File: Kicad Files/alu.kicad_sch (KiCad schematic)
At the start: 29 parts, among them U40 SST39SF040, U41 SST39SF040, U42 74LS173, U43 74HC245, U44 74HC245

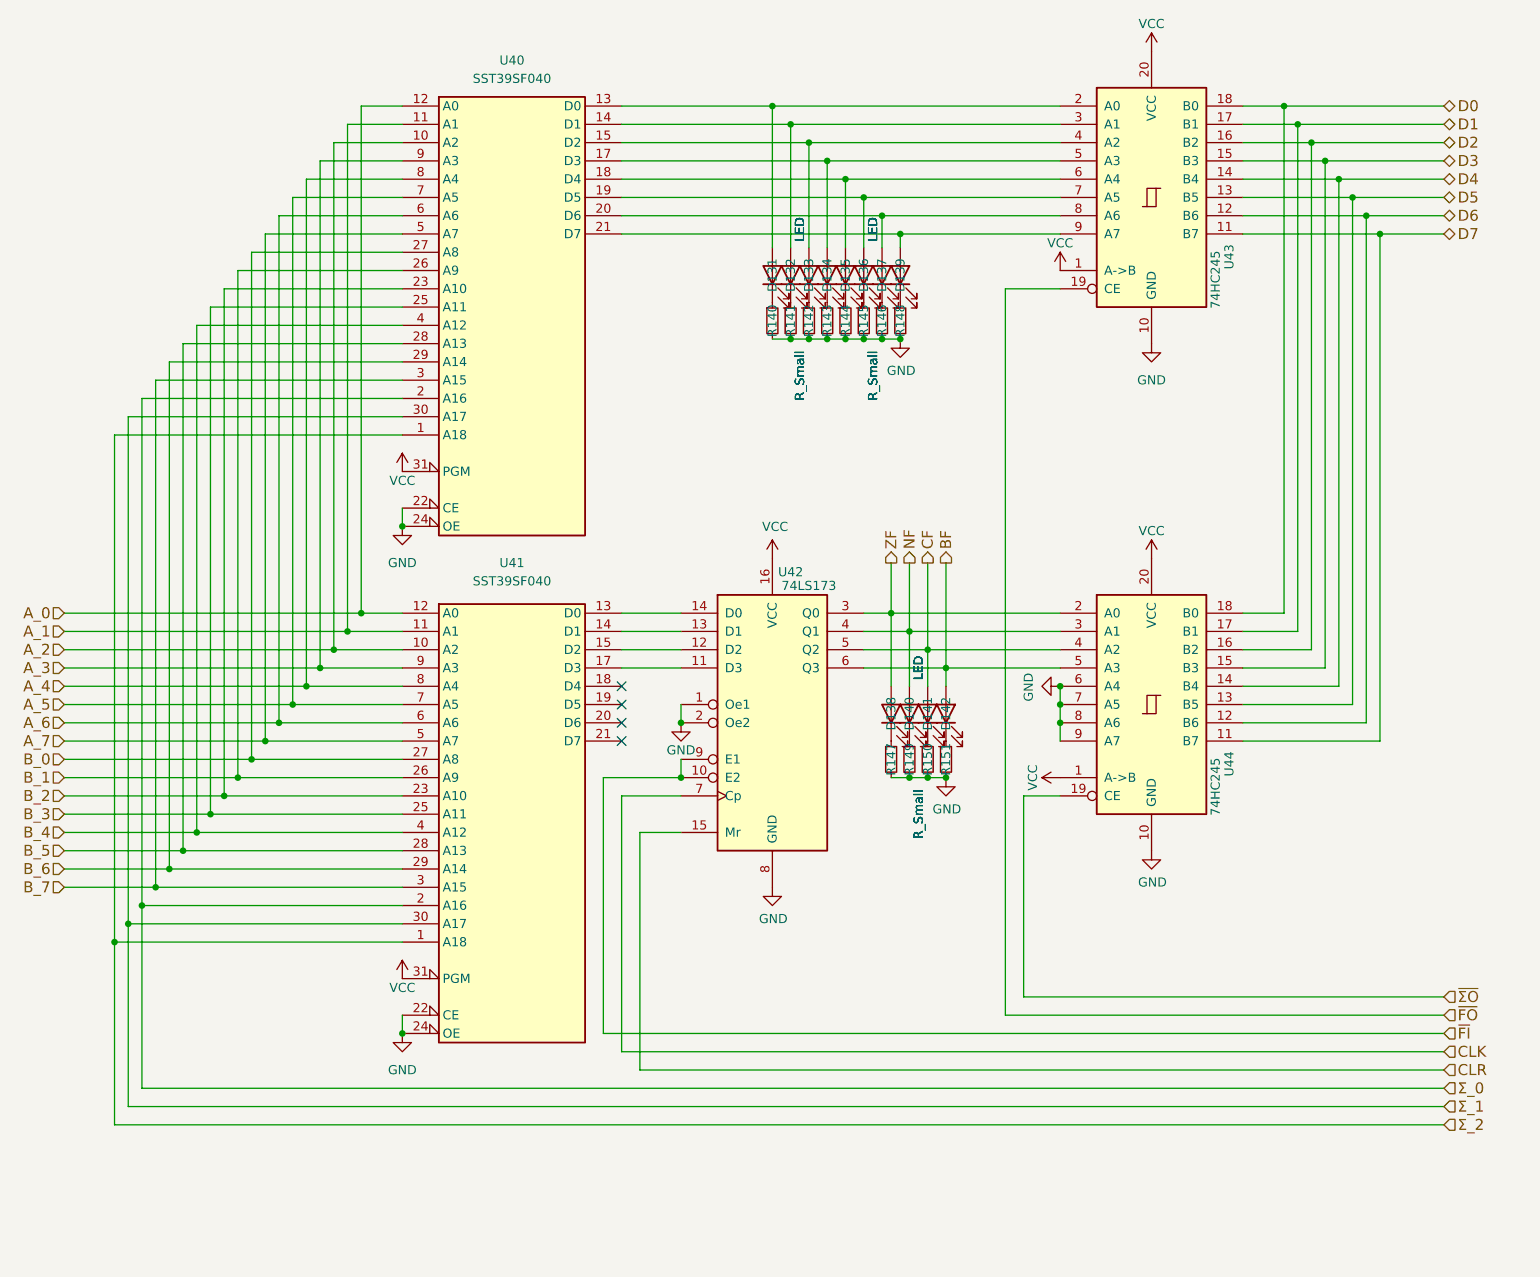
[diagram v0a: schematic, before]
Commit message: update
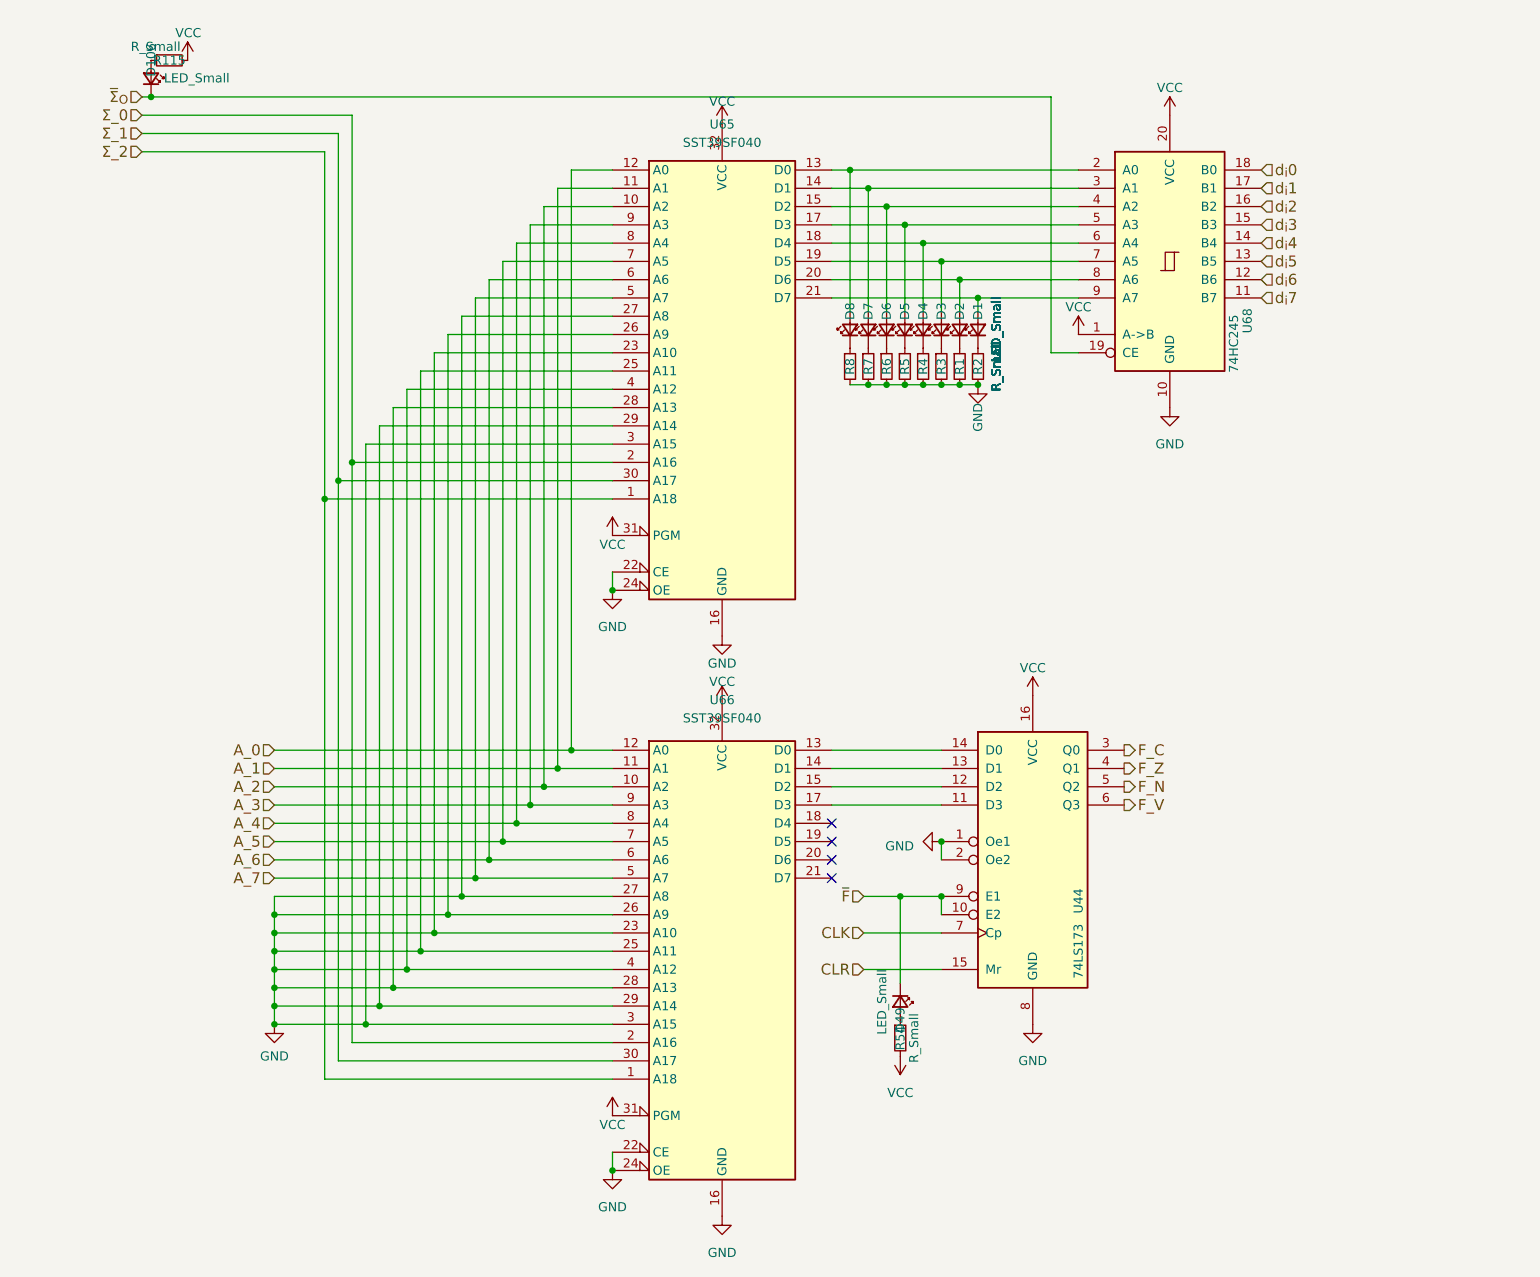
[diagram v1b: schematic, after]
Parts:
- removed D131, D132, D133, D134, D135, D136, D137, D138, D139, D140, D141, D142: LED, symbol Device:LED
- removed R140, R141, R142, R143, R144, R145, R146, R147, R148, R149, R150, R151: R_Small, symbol Device:R_Small
- removed U42: 74LS173, symbol 74xx:74LS173
- removed U44: 74HC245, symbol 74xx:74HC245
- added D1, D106, D2, D3, D4, D49, D5, D6, D7, D8: LED_Small, symbol Device:LED_Small
- added R1, R115, R2, R3, R4, R5, R54, R6, R7, R8: R_Small, symbol Device:R_Small
- added U44: 74LS173, symbol 74xx:74LS173
- renumbered U40 to U65, U41 to U66, U43 to U68
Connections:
- net B_0 is gone; now on net GND: U65.27 (A8), U66.27 (A8)
- net B_1 is gone; now on net GND: U65.26 (A9), U66.26 (A9)
- net B_2 is gone; now on net GND: U65.23 (A10), U66.23 (A10)
- net B_3 is gone; now on net GND: U65.25 (A11), U66.25 (A11)
- net B_4 is gone; now on net GND: U65.4 (A12), U66.4 (A12)
- net B_5 is gone; now on net GND: U65.28 (A13), U66.28 (A13)
- net B_6 is gone; now on net GND: U65.29 (A14), U66.29 (A14)
- net B_7 is gone; now on net GND: U65.3 (A15), U66.3 (A15)
- net CLK: now also U44.7 (Cp)
- net CLR: now also U44.15 (Mr)
- net GND: now also R1.2, R2.2, R3.2, R4.2, R5.2, R6.2, R7.2, R8.2, U44.1 (Oe1), U44.2 (Oe2), U44.8 (GND)
- net VCC: now also R115.2, R54.2, U44.16 (VCC)
- net at U65.15 (D2), U68.4 (A2): now also D6.2 (A)
- net at U65.19 (D5), U68.7 (A5): now also D3.2 (A)
- net at U65.13 (D0), U68.2 (A0): now also D8.2 (A)
- net at U65.17 (D3), U68.5 (A3): now also D5.2 (A)
- net at U66.17 (D3): now also U44.11 (D3)
- net at U66.15 (D2): now also U44.12 (D2)
- net at U66.14 (D1): now also U44.13 (D1)
- net at U66.13 (D0): now also U44.14 (D0)
- net at U65.21 (D7), U68.9 (A7): now also D1.2 (A)
- net at U65.14 (D1), U68.3 (A1): now also D7.2 (A)
- net at U65.18 (D4), U68.6 (A4): now also D4.2 (A)
- net at U65.20 (D6), U68.8 (A6): now also D2.2 (A)
- net D0 renamed d_{i}0
- net D1 renamed d_{i}1
- net D2 renamed d_{i}2
- net D3 renamed d_{i}3
- net D4 renamed d_{i}4
- net D5 renamed d_{i}5
- net D6 renamed d_{i}6
- net D7 renamed d_{i}7
- net ~{FO} renamed ~{Σ}_{O}
- net ~{Σ}_{O}: now also D106.1 (K)
- new net: D8.1 (K), R8.1
- new net: D1.1 (K), R2.1
- new net: D4.1 (K), R4.1
- new net: D3.1 (K), R3.1
- new net: D5.1 (K), R5.1
- new net: D2.1 (K), R1.1
- new net: D6.1 (K), R6.1
- new net: D106.2 (A), R115.1
- new net: D49.2 (A), R54.1
- new net: D7.1 (K), R7.1
- new net F_C: U44.3 (Q0)
- new net F_N: U44.5 (Q2)
- new net F_V: U44.6 (Q3)
- new net F_Z: U44.4 (Q1)
- new net ~{F}: D49.1 (K), U44.10 (E2), U44.9 (E1)
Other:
- moved on the sheet: U68
